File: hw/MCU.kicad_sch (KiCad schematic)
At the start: 3 parts, among them IC3 STM32G071RBT6, J1 Conn_ARM_JTAG_SWD_10

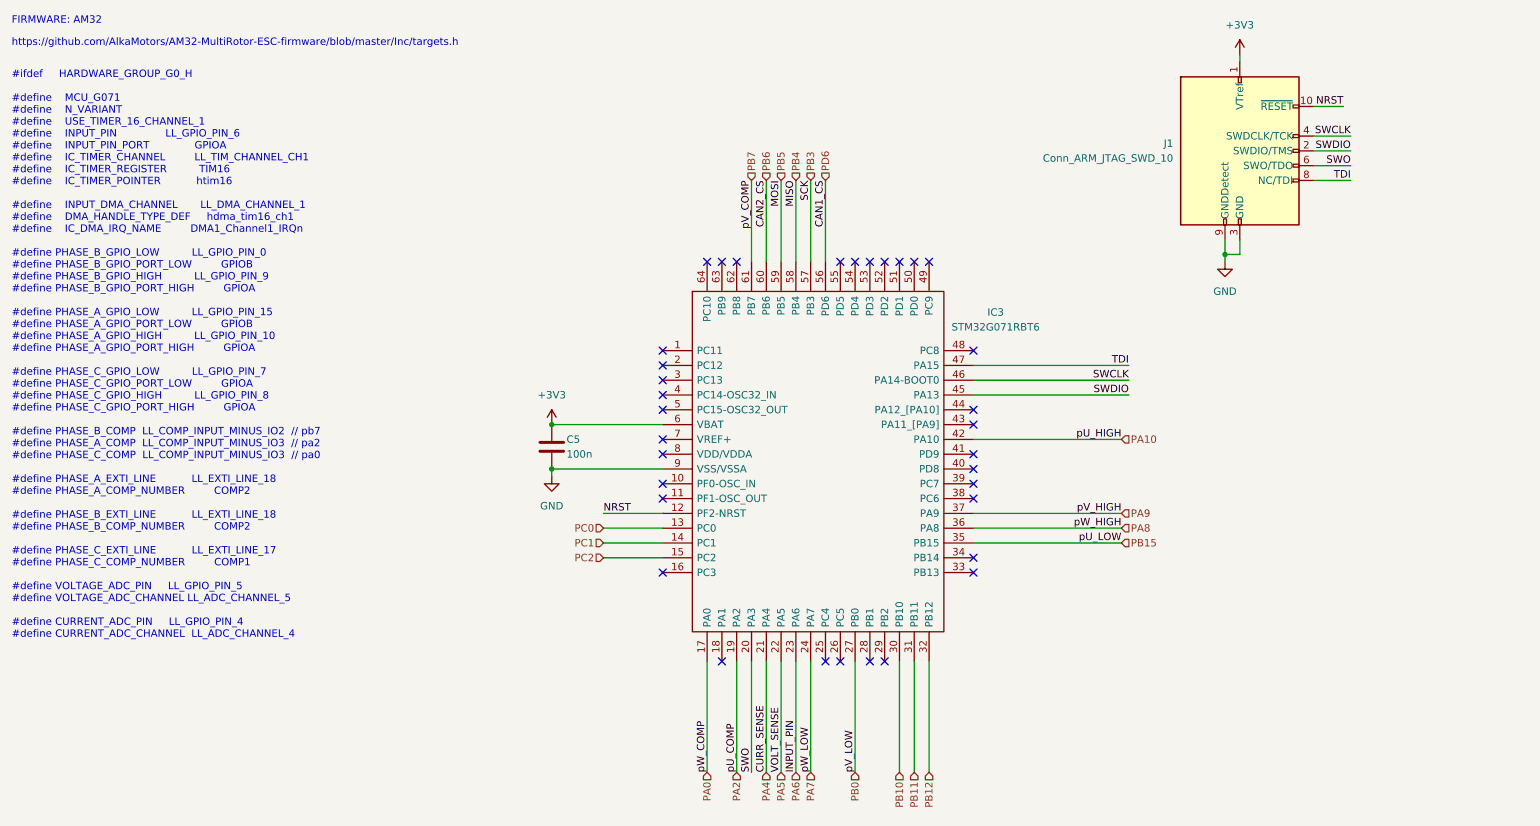
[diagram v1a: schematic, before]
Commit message: commenting
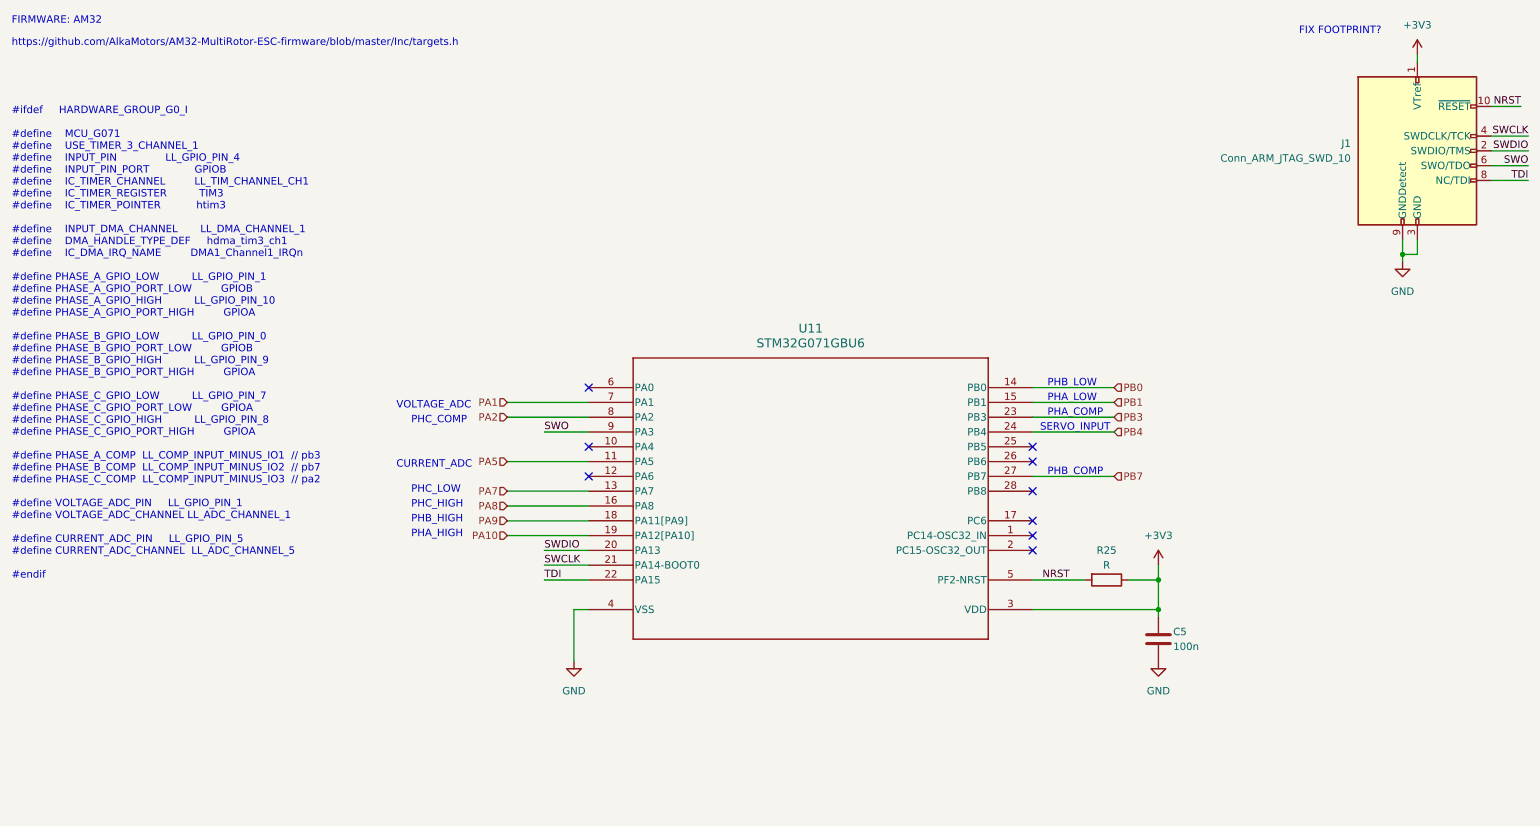
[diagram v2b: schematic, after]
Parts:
- removed IC3: STM32G071RBT6, QFP50P1200X1200X160-64N, symbol MAG_MCUs:STM32G071RBT6
- added R25: R, symbol Device:R
- added U11: STM32G071GBU6, UFQFPN-28, symbol MAG_MCUs:STM32G071GBU6
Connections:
- net +3V3: now also R25.1, U11.3 (VDD)
- net GND: now also U11.4 (VSS)
- net NRST: now also R25.2, U11.5 (PF2-NRST)
- net PA10: now also U11.19 (PA12[PA10])
- net PA2: now also U11.8 (PA2)
- net PA5: now also U11.11 (PA5)
- net PA7: now also U11.13 (PA7)
- net PA8: now also U11.16 (PA8)
- net PA9: now also U11.18 (PA11[PA9])
- net PB0: now also U11.14 (PB0)
- net PB3: now also U11.23 (PB3)
- net PB4: now also U11.24 (PB4)
- net PB7: now also U11.27 (PB7)
- net SWCLK: now also U11.21 (PA14-BOOT0)
- net SWDIO: now also U11.20 (PA13)
- net SWO: now also U11.9 (PA3)
- net TDI: now also U11.22 (PA15)
- new net PA1: U11.7 (PA1)
- new net PB1: U11.15 (PB1)
- no-connect marks 34 -> 9
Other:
- note added: "#ifdef HARDWARE_GROUP_G0_I #define MCU_G071 #define USE_TIMER_3_CHANNEL_1 #define INPUT_PIN LL_GPIO_PIN_4 #define INPUT_PIN_PORT GPIOB #define IC_TIMER_CHANNEL LL_TIM_CHANNEL_CH1 #define IC_TIMER_REGISTER TIM3 #define IC_TIMER_POINTER htim3 #define INPUT_DMA_CHANNEL LL_DMA_CHANNEL_1 #define DMA_HANDLE_TYPE_DEF hdma_tim3_ch1 #define IC_DMA_IRQ_NAME DMA1_Channel1_IRQn #define PHASE_A_GPIO_LOW LL_GP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"
- note added: "CURRENT_ADC"
- note added: "FIX FOOTPRINT?"
- note added: "PHA_COMP"
- note added: "PHA_HIGH"
- note added: "PHA_LOW"
- note added: "PHB_COMP"
- note added: "PHB_HIGH"
- note added: "PHB_LOW"
- note added: "PHC_COMP"
- note added: "PHC_HIGH"
- note added: "PHC_LOW"
- note added: "SERVO_INPUT"
- note added: "VOLTAGE_ADC"
- note removed: "#ifdef HARDWARE_GROUP_G0_H #define MCU_G071 #define N_VARIANT #define USE_TIMER_16_CHANNEL_1 #define INPUT_PIN LL_GPIO_PIN_6 #define INPUT_PIN_PORT GPIOA #define IC_TIMER_CHANNEL LL_TIM_CHANNEL_CH1 #define IC_TIMER_REGISTER TIM16 #define IC_TIMER_POINTER htim16 #define INPUT_DMA_CHANNEL LL_DMA_CHANNEL_1 #define DMA_HANDLE_TYPE_DEF hdma_tim16_ch1 #define IC_DMA_IRQ_NAME DMA1_Channel1_IRQn #define 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"
- moved on the sheet: C5, J1
